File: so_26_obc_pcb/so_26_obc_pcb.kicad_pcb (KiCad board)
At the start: 4 copper layers, 90.2 x 95.9 mm, 52 parts, among them J1 Conn_02x06_Odd_Even, J2 Conn_02x12_Odd_Even, J3 Conn_01x04, J4 Conn_01x03, J5 Conn_01x02, J6 Conn_01x02, J7 Conn_01x02, J8 Conn_01x03, J9 Conn_01x03, SW1 SW_Push, U1 STM32G431RBTx, U2 TPT3232A-TS3R, U3 PCT2075, U4 MPRLS0025, U5 LSM6DS3, U6 MEM2067-02-180-00-A

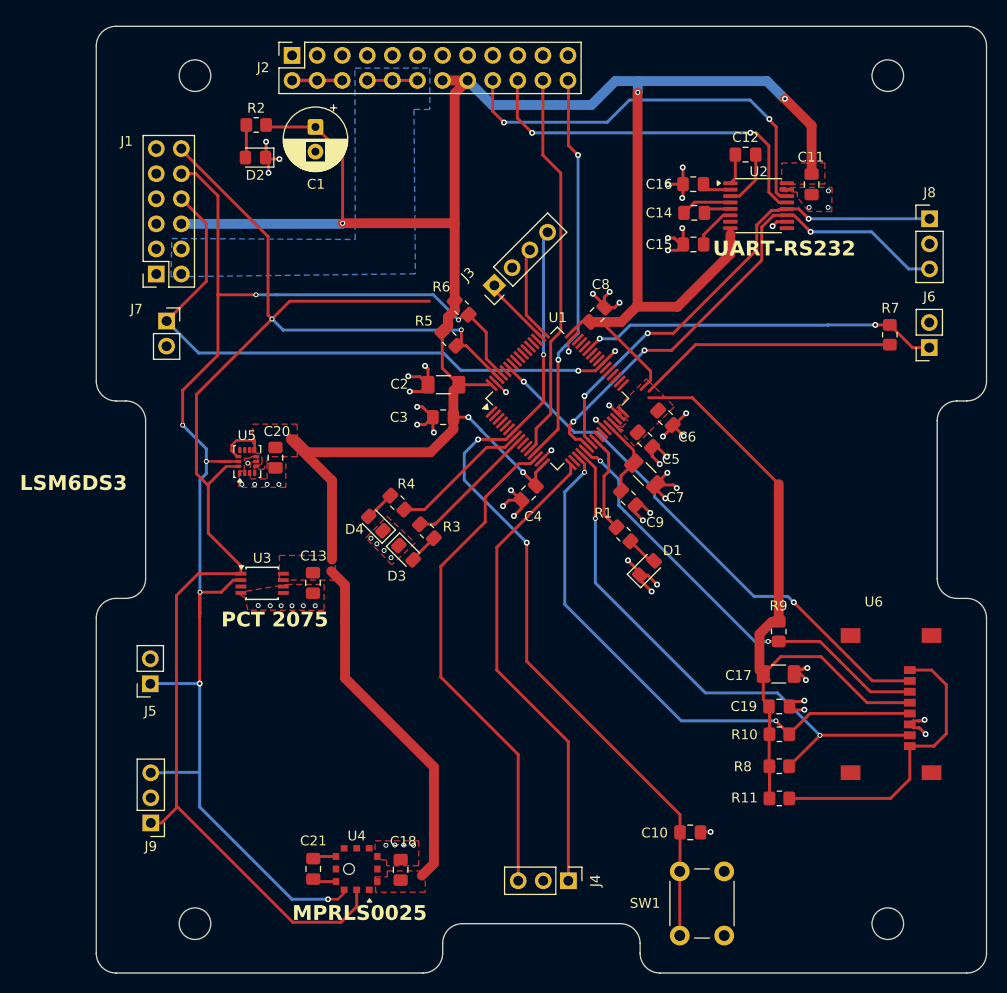
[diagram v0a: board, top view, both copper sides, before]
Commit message: PCB: final routing + review
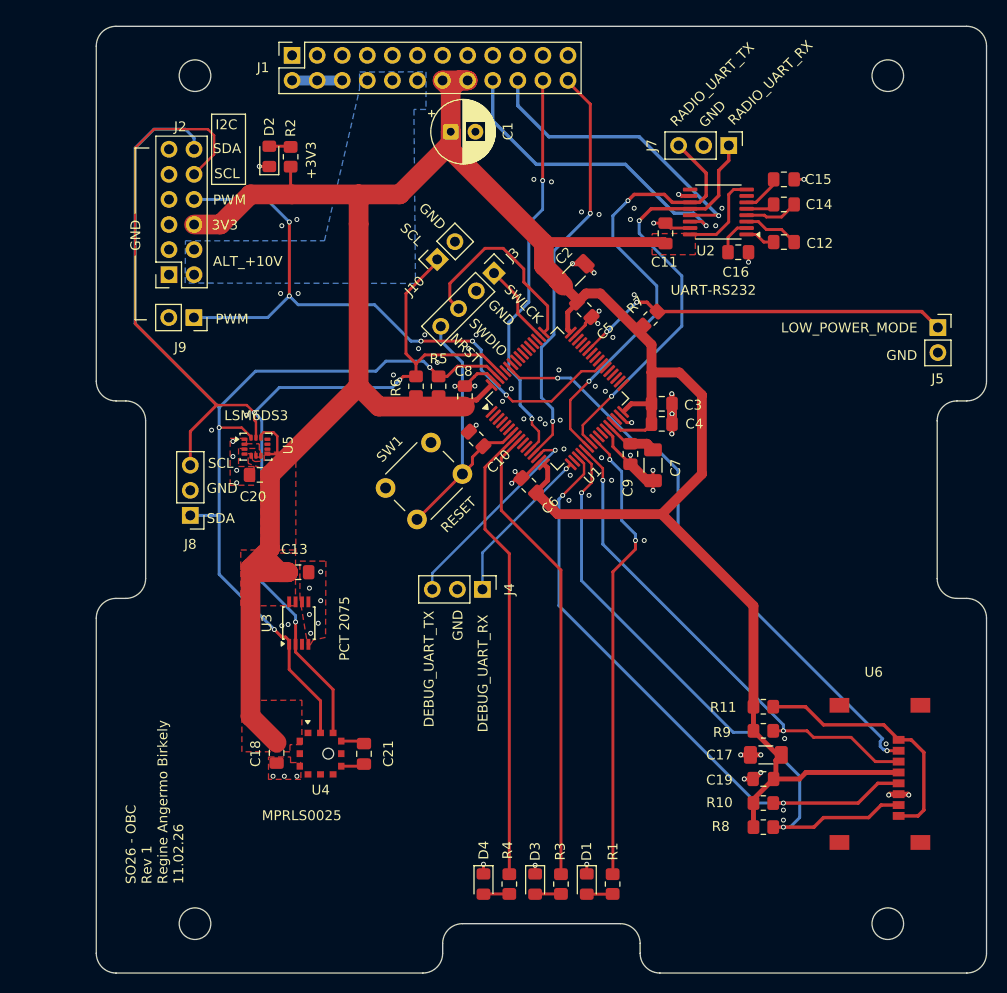
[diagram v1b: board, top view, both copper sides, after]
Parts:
- moved J10 51.9 mm to (90.5, 68.9), turned to 135 degrees
- moved SW1 51.7 mm to (93.1, 90.7), turned to -135 degrees
- moved C10 45.4 mm to (94.5, 87.1), turned to 135 degrees
- moved R4 40.3 mm to (97.8, 132.2), turned to 90 degrees
- moved R3 38.2 mm to (103.1, 132.2), turned to 90 degrees
- moved D4 38.1 mm to (95.2, 132.2), turned to -90 degrees
- moved D3 36.0 mm to (100.5, 132.2), turned to -90 degrees
- moved R1 35.5 mm to (108.3, 132.2), turned to 90 degrees
- moved D1 32.6 mm to (105.7, 132.2), turned to -90 degrees
- moved J8 31.4 mm to (65.5, 94.8)
- moved J4 30.8 mm to (95.1, 102.3)
- moved R7 24.3 mm to (112.1, 74.9), turned to -135 degrees
- moved C3 22.2 mm to (113.3, 83.5), turned to 0 degrees
- moved J7 21.7 mm to (120.1, 57.4), turned to -90 degrees
- moved C2 17.3 mm to (104.4, 70.5), turned to 45 degrees
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- renumbered J2 to J1, J5 to J10, J1 to J2, J6 to J5, J8 to J7, J9 to J8, J7 to J9
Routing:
- net +3V3: track 375.4 -> 294.5 mm, vias 5 -> 0
- net /NRST: track 85.4 -> 29.6 mm, vias 3 -> 0
- net /I2C_SDA: track 157.2 -> 114.0 mm, vias 2 -> 3
- net /LED_BLUE: track 10.1 -> 46.6 mm, vias 0 -> 2
- net /LED_YELLOW: track 13.6 -> 47.3 mm
- net /LED_GREEN: track 14.4 -> 46.7 mm
- net /DEBUG_UART_RX: track 48.3 -> 16.4 mm, vias 0 -> 1
- net GND: track 83.8 -> 52.7 mm, vias 69 -> 87
- net /DEBUG_UART_TX: track 50.9 -> 21.4 mm, vias 0 -> 1
- net /SWDIO: track 9.27 -> 20.4 mm
- net /RADIO_TX: track 42.3 -> 31.9 mm, vias 2 -> 1
- net /BOOT0: track 143.8 -> 134.4 mm, vias 7 -> 3
- net /SD_MISO: track 56.9 -> 63.9 mm
- net /RADIO_RX: track 37.4 -> 30.4 mm, vias 2 -> 1
- net /RADIO_UART_RX: track 49.9 -> 43.5 mm, vias 3 -> 2
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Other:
- board text added: "+3V3"
- board text added: "3V3"
- board text added: "ALT_+10V"
- board text added: "DEBUG_UART_RX"
- board text added: "DEBUG_UART_TX"
- board text added: "GND"
- board text added: "I2C"
- board text added: "LOW_POWER_MODE"
- board text added: "NRST"
- board text added: "PWM"
- board text added: "RADIO_UART_RX"
- board text added: "RADIO_UART_TX"
- board text added: "RESET"
- board text added: "SCL"
- board text added: "SDA"
- board text added: "SO26 - OBC Rev 1 Regine Angermo Birkely 11.02.26"
- board text added: "SWDIO"
- board text added: "SWLCK"
- board text removed: "Regine Angermo Birkely SubOrbital 25/26 Orbit NTNU"
- board text removed: "SO_25/26_ OBC_PCB 11.02.26 Rev. 1"
